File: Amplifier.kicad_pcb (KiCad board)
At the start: 2 copper layers, 63 x 100 mm, 28 parts, among them J1 Input, J2 Conn_01x04, J3 output, J4 Neon bulb, T1 Transformer_SP_1S, U1 6N2P, U2 6P14P

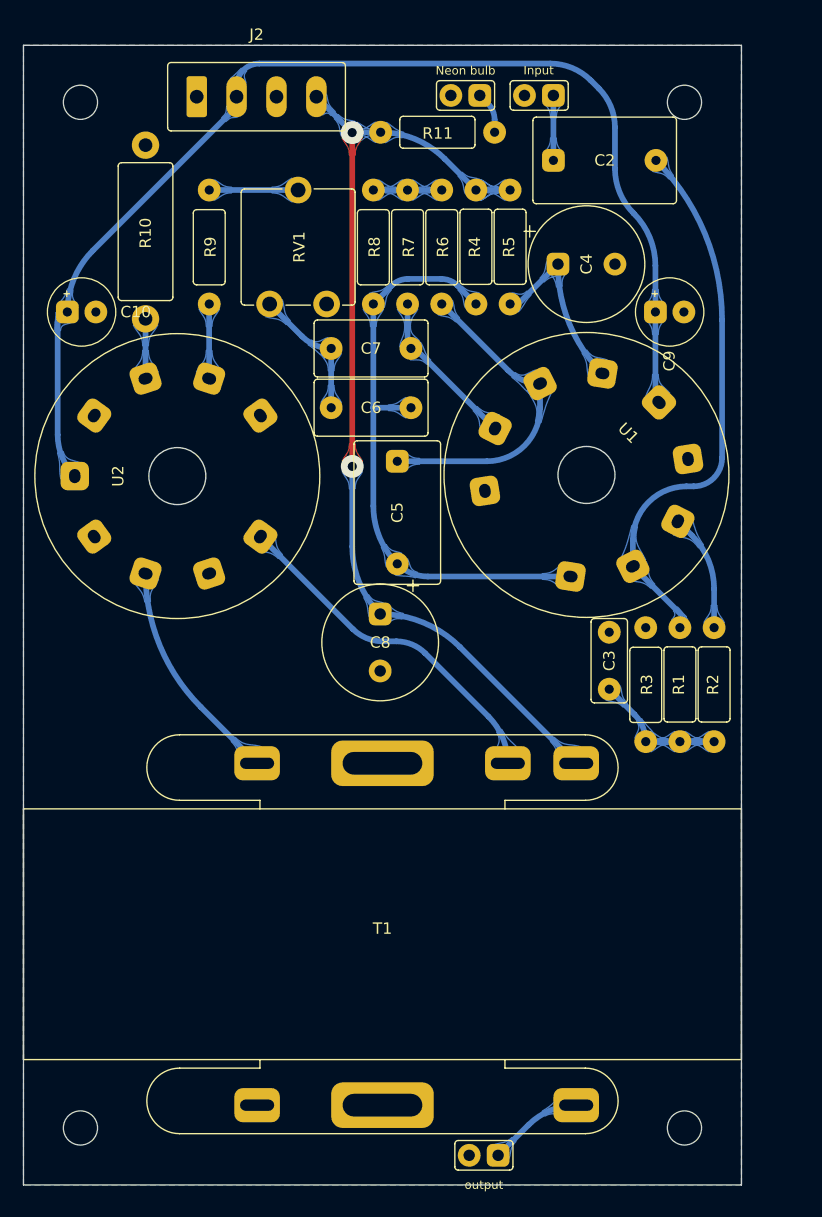
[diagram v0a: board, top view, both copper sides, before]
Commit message: Temp
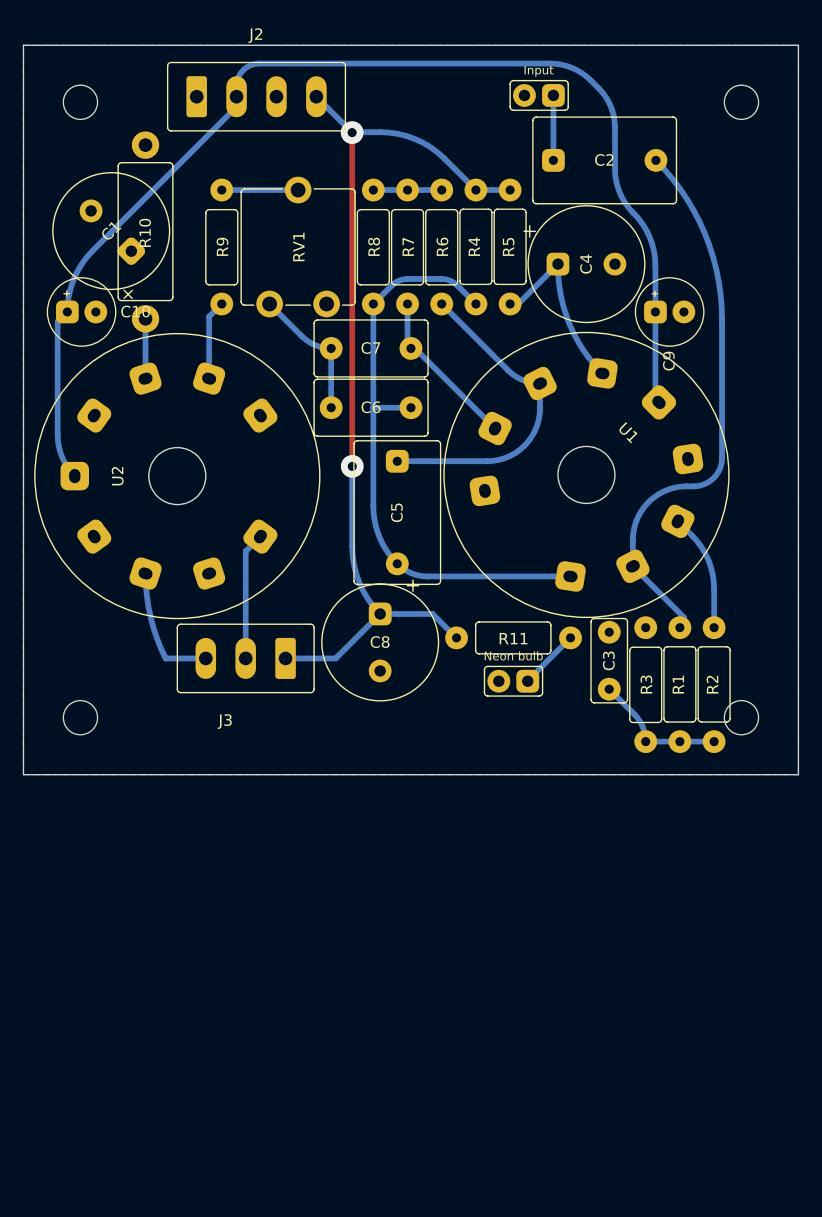
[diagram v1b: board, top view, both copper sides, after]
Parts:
- removed T1: Transformer_SP_1S, spdf1626_lib:Output_transformer
- added C1: 10uF, spdf1626_lib:C_THT_D10.0mm_P5.00mm, F.Cu at (64.7, 56.3)
- J2: value Conn_01x04 -> Power
- J3: value output -> Transformer; footprint spdf1626_lib:PinHeader_1x02_P2.54mm -> spdf1626_lib:MCV_1,5_4-G-3.5_1x03_P3.50mm_Vertical
- moved J4 51.6 mm to (101.2, 95.8)
- moved J3 48.9 mm to (76.5, 93.8), turned to 180 degrees
- moved R11 44.9 mm to (100.0, 92.0)
- moved R9 1.10 mm to (74.4, 57.7)
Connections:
- J3 pad 1: Left_output -> 240V
- J3 pad 2: GND -> Net-(U2-Pad9)
- U2 pad 7: Net-(T1-Pad3) -> Net-(U2-Pad7)
- U2 pad 9: Net-(T1-Pad2) -> Net-(U2-Pad9)
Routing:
- net Net-(T1-Pad2): track 30.7 -> 0.00 mm
- net Net-(T1-Pad3): track 19.9 -> 0.00 mm
- net Net-(U2-Pad7): track 0.00 -> 11.2 mm
- net Net-(U2-Pad9): track 0.00 -> 11.2 mm
- net Left_output: track 8.39 -> 0.00 mm
- net 240V: track 85.1 -> 80.4 mm
- net Net-(J4-Pad1): track 3.67 -> 5.35 mm
- net Net-(R9-Pad1): track 7.80 -> 6.70 mm
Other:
- board size 63 x 100 mm -> 68 x 64 mm
